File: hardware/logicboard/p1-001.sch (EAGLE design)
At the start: 25 parts, among them IC1 74LS07N

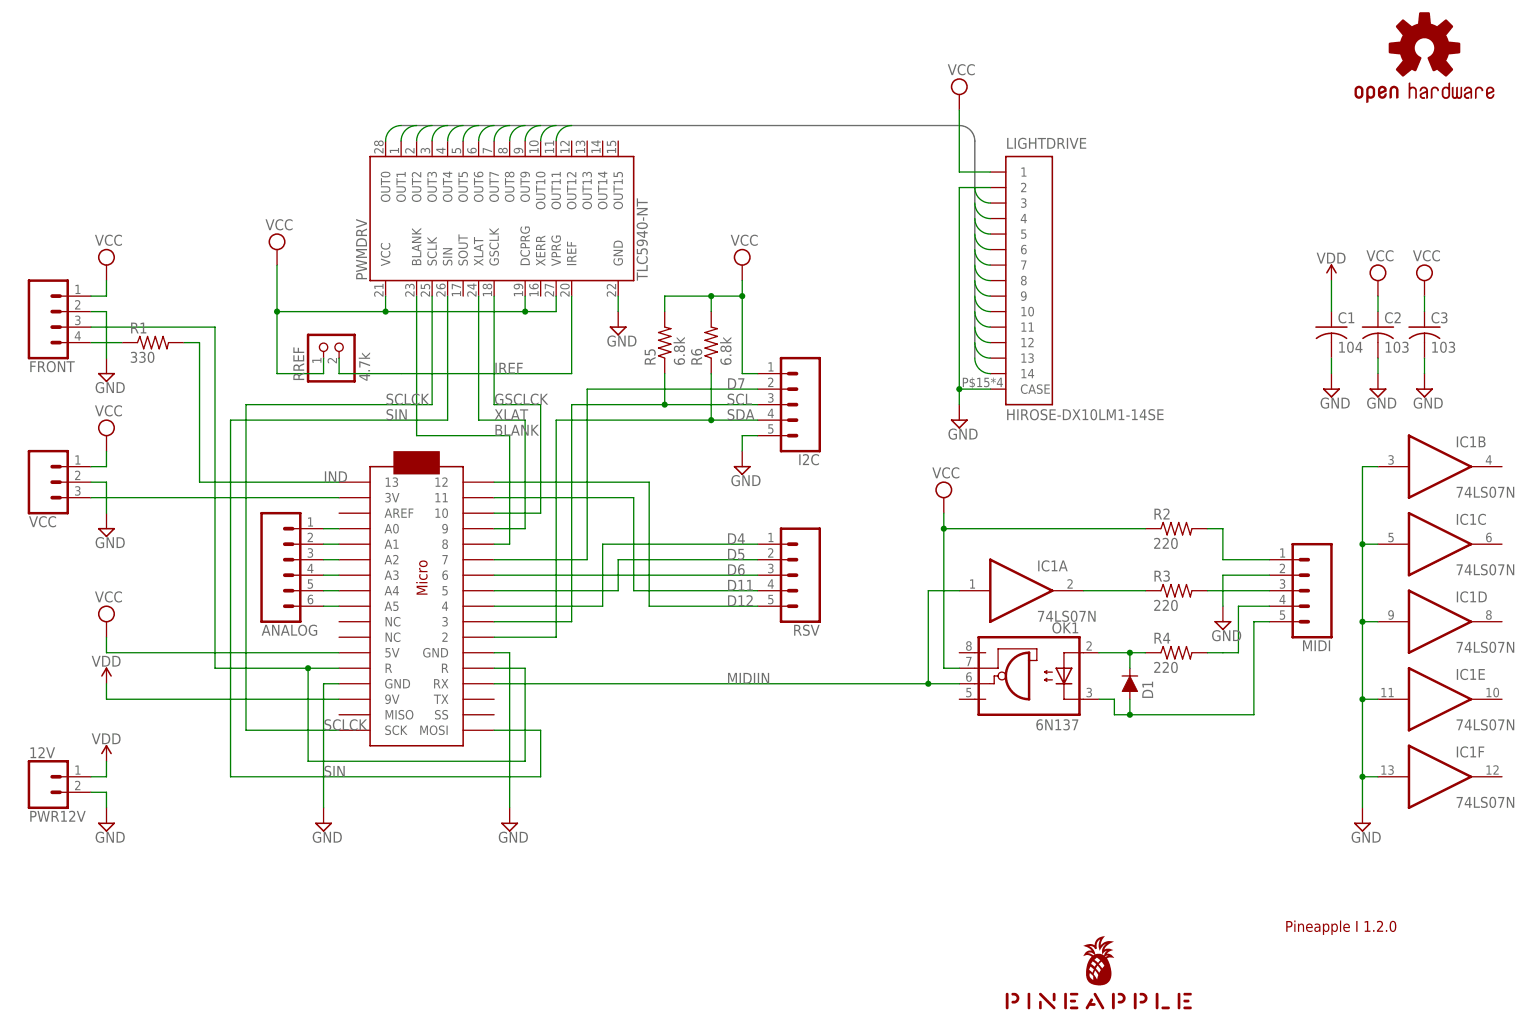
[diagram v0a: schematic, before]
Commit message: New design.
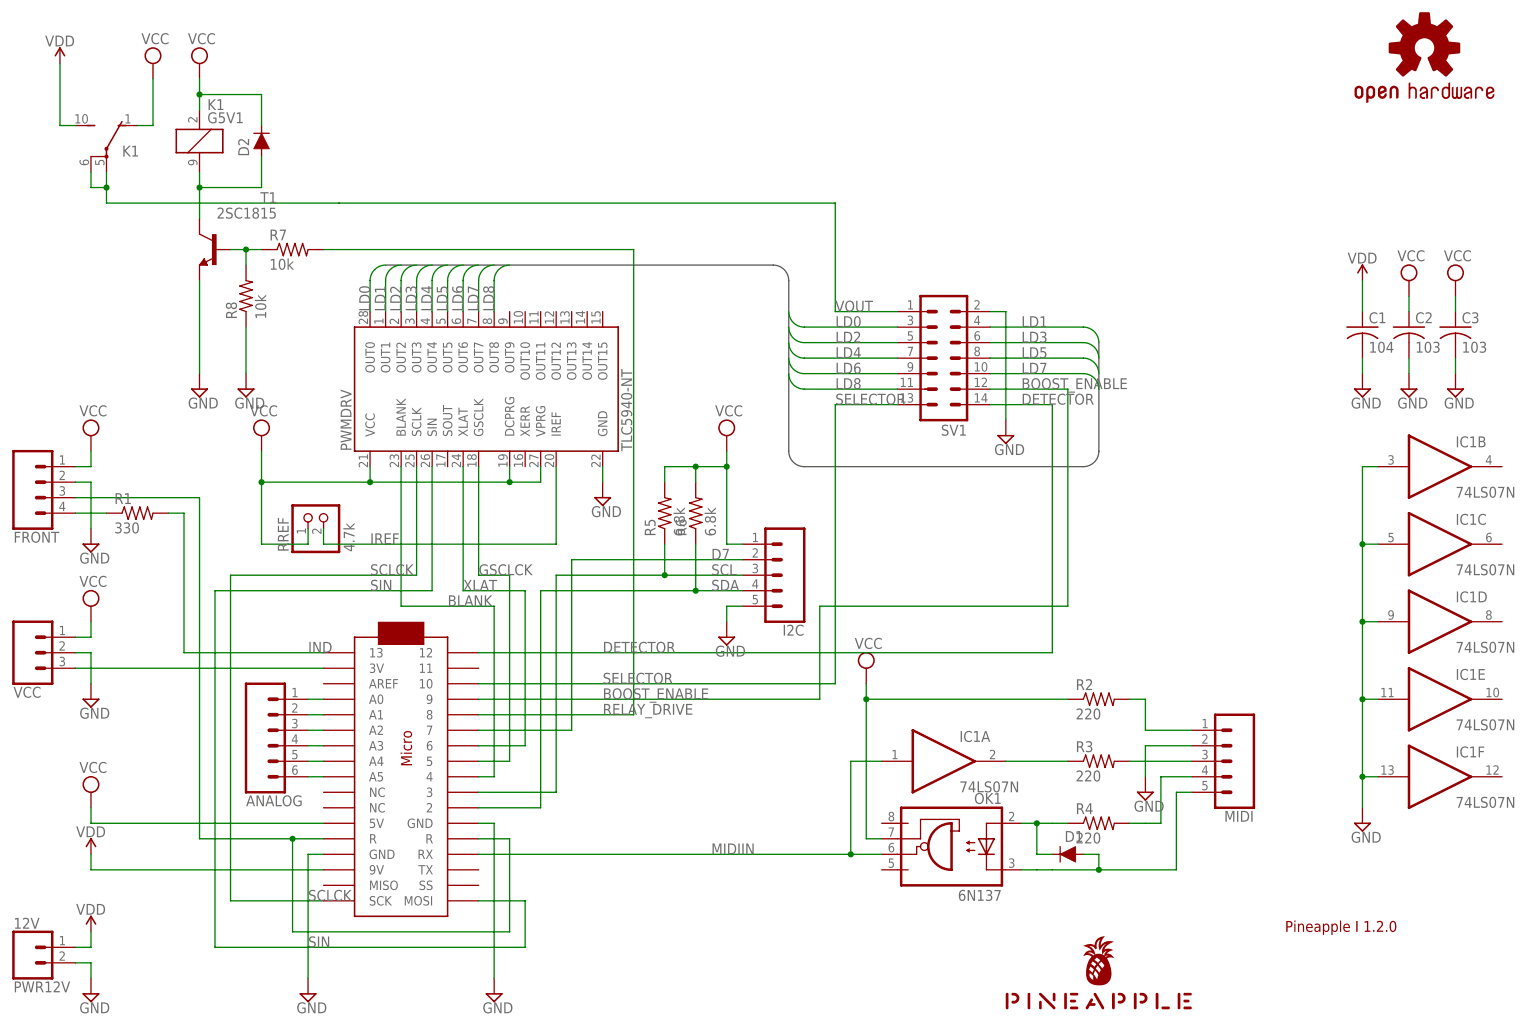
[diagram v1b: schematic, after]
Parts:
- removed LIGHTDRIVE: HIROSE-DX10LM1-14SE, con-hirose-dx10lm1-14se:HIROSE-DX10LM1-14SE
- removed RSV: (no value), SparkFun-Connectors:CONN_051.27MM
- added D2: DIODE-1N4148, SparkFun-DiscreteSemi:DIODE-1N4148
- added K1: G5V1, relay:G5V1
- added R7, R8: 10k, resistor:R-US_0204/5
- added SV1: (no value), con-ml:ML14L
- added T1: 2SC1815, transistor:2SC1815
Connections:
- removed net D11: RSV.4, U$1.11
- removed net D12: RSV.5, U$1.12
- removed net D4: RSV.1, U$1.4
- removed net D5: RSV.2, U$1.5
- removed net D6: RSV.3, U$1.6
- removed net LD10: LIGHTDRIVE.12, PWMDRV.OUT9
- removed net LD11: LIGHTDRIVE.13, PWMDRV.OUT10
- removed net LD12: LIGHTDRIVE.14, PWMDRV.OUT11
- removed net LD9: LIGHTDRIVE.11, PWMDRV.OUT8
- new net BOOST_ENABLE: SV1.12, U$1.9
- new net DETECTOR: SV1.14, U$1.12
- new net LD0: PWMDRV.OUT0, SV1.3
- new net N$2: R7.1, R8.2, T1.B
- new net N$3: D2.A, K11.2, T1.C
- new net RELAY_DRIVE: R7.2, U$1.8
- new net SELECTOR: SV1.13, U$1.10
- new net VOUT: K12.P, K12.P@1, SV1.1
- net BLANK: now also U$1.4; no longer U$1.8
- net GND: now also R8.1, SV1.2, T1.E; no longer LIGHTDRIVE.2, LIGHTDRIVE.CASE
- net GSCLCK: now also U$1.5; no longer U$1.10
- net LD1: now also PWMDRV.OUT1, SV1.4; no longer LIGHTDRIVE.3, PWMDRV.OUT0
- net LD2: now also PWMDRV.OUT2, SV1.5; no longer LIGHTDRIVE.4, PWMDRV.OUT1
- net LD3: now also PWMDRV.OUT3, SV1.6; no longer LIGHTDRIVE.5, PWMDRV.OUT2
- net LD4: now also PWMDRV.OUT4, SV1.7; no longer LIGHTDRIVE.6, PWMDRV.OUT3
- net LD5: now also PWMDRV.OUT5, SV1.8; no longer LIGHTDRIVE.7, PWMDRV.OUT4
- net LD6: now also PWMDRV.OUT6, SV1.9; no longer LIGHTDRIVE.8, PWMDRV.OUT5
- net LD7: now also PWMDRV.OUT7, SV1.10; no longer LIGHTDRIVE.9, PWMDRV.OUT6
- net LD8: now also PWMDRV.OUT8, SV1.11; no longer LIGHTDRIVE.10, PWMDRV.OUT7
- net VCC: now also D2.C, K11.1, K12.O; no longer LIGHTDRIVE.1
- net VDD: now also K12.S
- net XLAT: now also U$1.6; no longer U$1.9
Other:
- moved on the sheet: ANALOG, C1, C2, C3, D1, FRONT, I2C, IC1A, MIDI, OK1, PWMDRV, PWR12V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
